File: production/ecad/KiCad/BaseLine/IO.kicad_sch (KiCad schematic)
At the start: 5 parts, among them J10 Conn_LoadCell1, J11 Conn_LoadCell2, J12 Conn_LoadCell3, J13 Conn_LoadCell4, U12 CD74HC4067M96

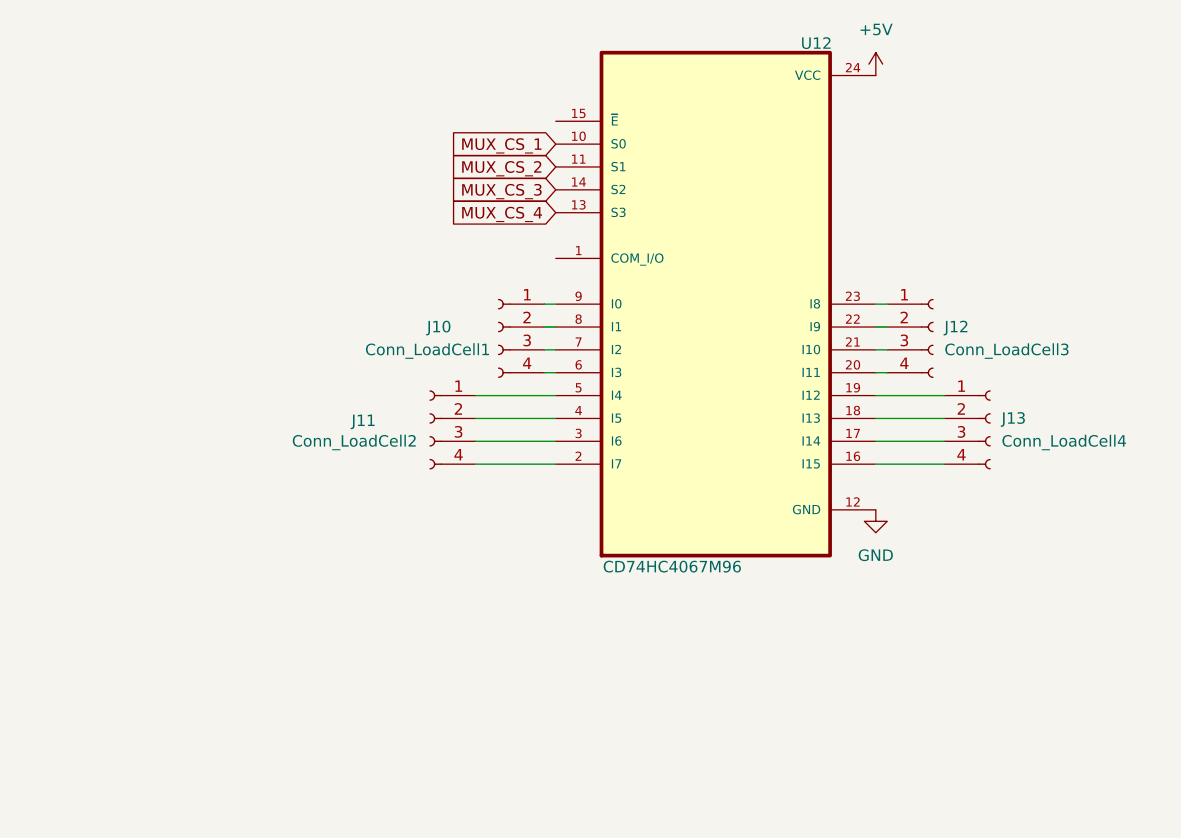
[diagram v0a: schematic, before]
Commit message: Final mux changes
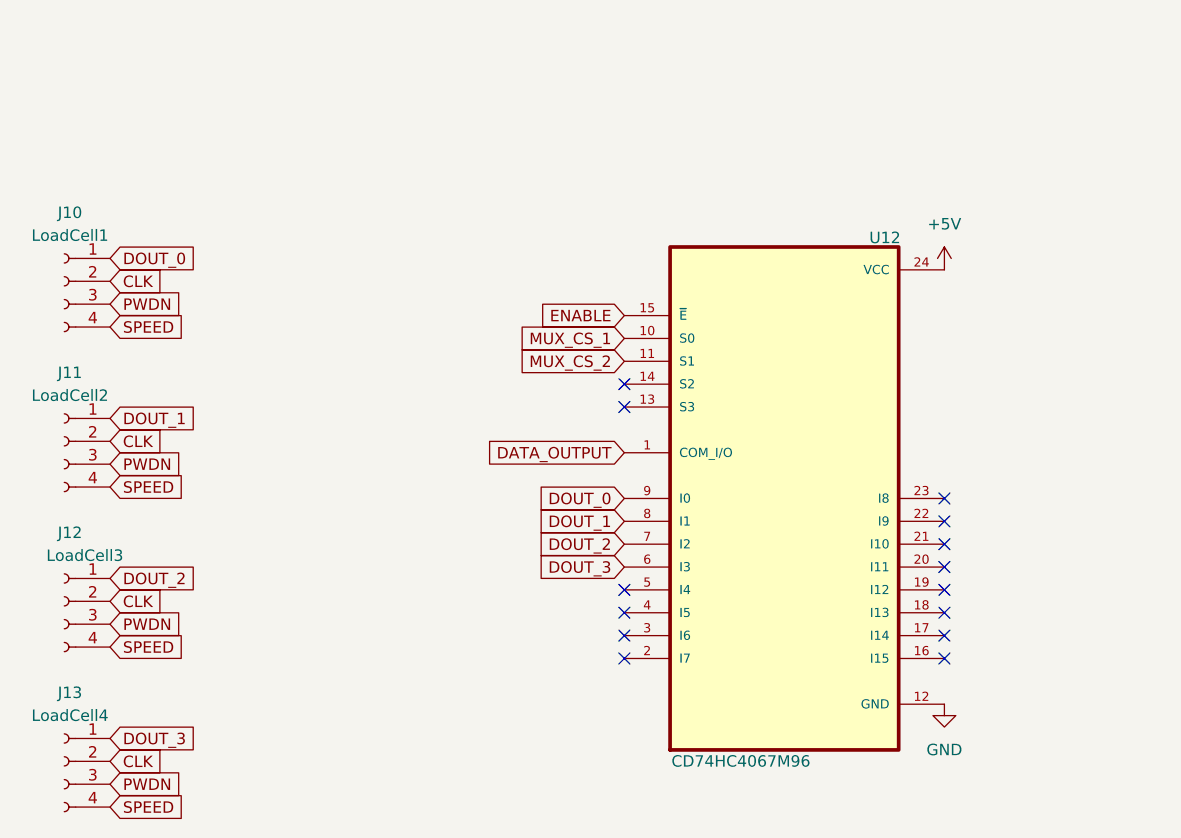
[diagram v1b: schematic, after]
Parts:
- J10: value Conn_LoadCell1 -> LoadCell1
- J11: value Conn_LoadCell2 -> LoadCell2
- J12: value Conn_LoadCell3 -> LoadCell3
- J13: value Conn_LoadCell4 -> LoadCell4
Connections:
- net DATA_OUTPUT: now reaches U12.1 (COM_I/O)
- net ENABLE: now reaches U12.15 (~{E})
- net at U12.16 (I15): no longer J13.4 (Pin_4)
- net at U12.17 (I14): no longer J13.3 (Pin_3)
- net at U12.18 (I13): no longer J13.2 (Pin_2)
- net at U12.19 (I12): no longer J13.1 (Pin_1)
- net at U12.2 (I7): no longer J11.4 (Pin_4)
- net at U12.20 (I11): no longer J12.4 (Pin_4)
- net at U12.21 (I10): no longer J12.3 (Pin_3)
- net at U12.22 (I9): no longer J12.2 (Pin_2)
- net at U12.23 (I8): no longer J12.1 (Pin_1)
- net at U12.3 (I6): no longer J11.3 (Pin_3)
- net at U12.4 (I5): no longer J11.2 (Pin_2)
- net at U12.5 (I4): no longer J11.1 (Pin_1)
- net DOUT_3: now reaches U12.6 (I3)
- net DOUT_3: now also J13.1 (Pin_1); no longer J10.4 (Pin_4)
- net DOUT_2: now reaches U12.7 (I2)
- net DOUT_2: now also J12.1 (Pin_1); no longer J10.3 (Pin_3)
- net CLK: now reaches J10.2 (Pin_2)
- net CLK: now also J11.2 (Pin_2), J12.2 (Pin_2), J13.2 (Pin_2); no longer U12.8 (I1)
- net DOUT_0: now reaches J10.1 (Pin_1), U12.9 (I0)
- net MUX_CS_3: no longer names the net of U12.14 (S2)
- net MUX_CS_4: no longer names the net of U12.13 (S3)
- new net DOUT_1: J11.1 (Pin_1), U12.8 (I1)
- new net PWDN: J10.3 (Pin_3), J11.3 (Pin_3), J12.3 (Pin_3), J13.3 (Pin_3)
- new net SPEED: J10.4 (Pin_4), J11.4 (Pin_4), J12.4 (Pin_4), J13.4 (Pin_4)
- no-connect marks 0 -> 14
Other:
- moved on the sheet: U12
